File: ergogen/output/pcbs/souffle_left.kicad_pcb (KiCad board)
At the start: 2 copper layers, 135.6 x 116.1 mm, 60 parts

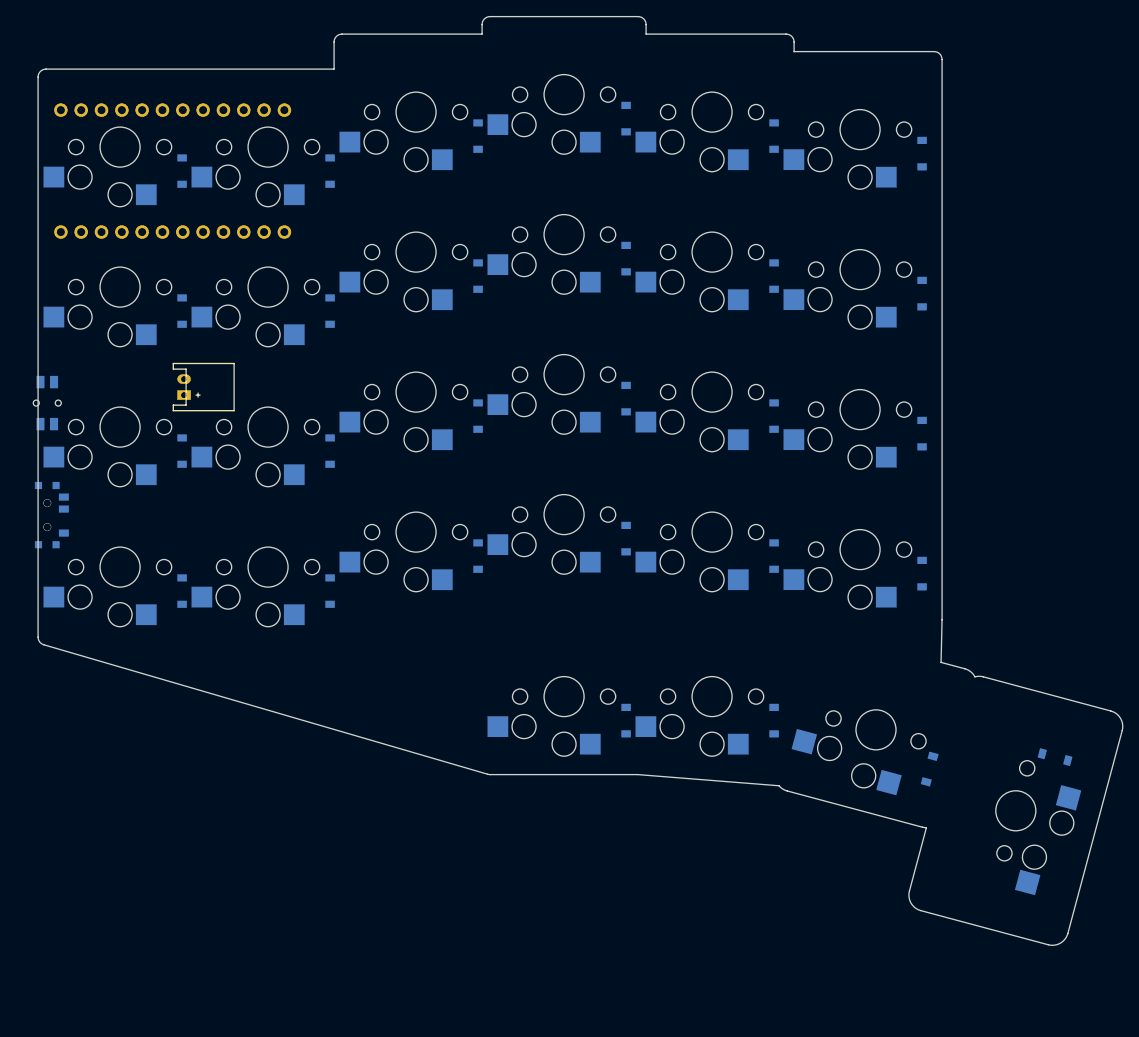
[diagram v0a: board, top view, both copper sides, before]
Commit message: feat: left hand redesign
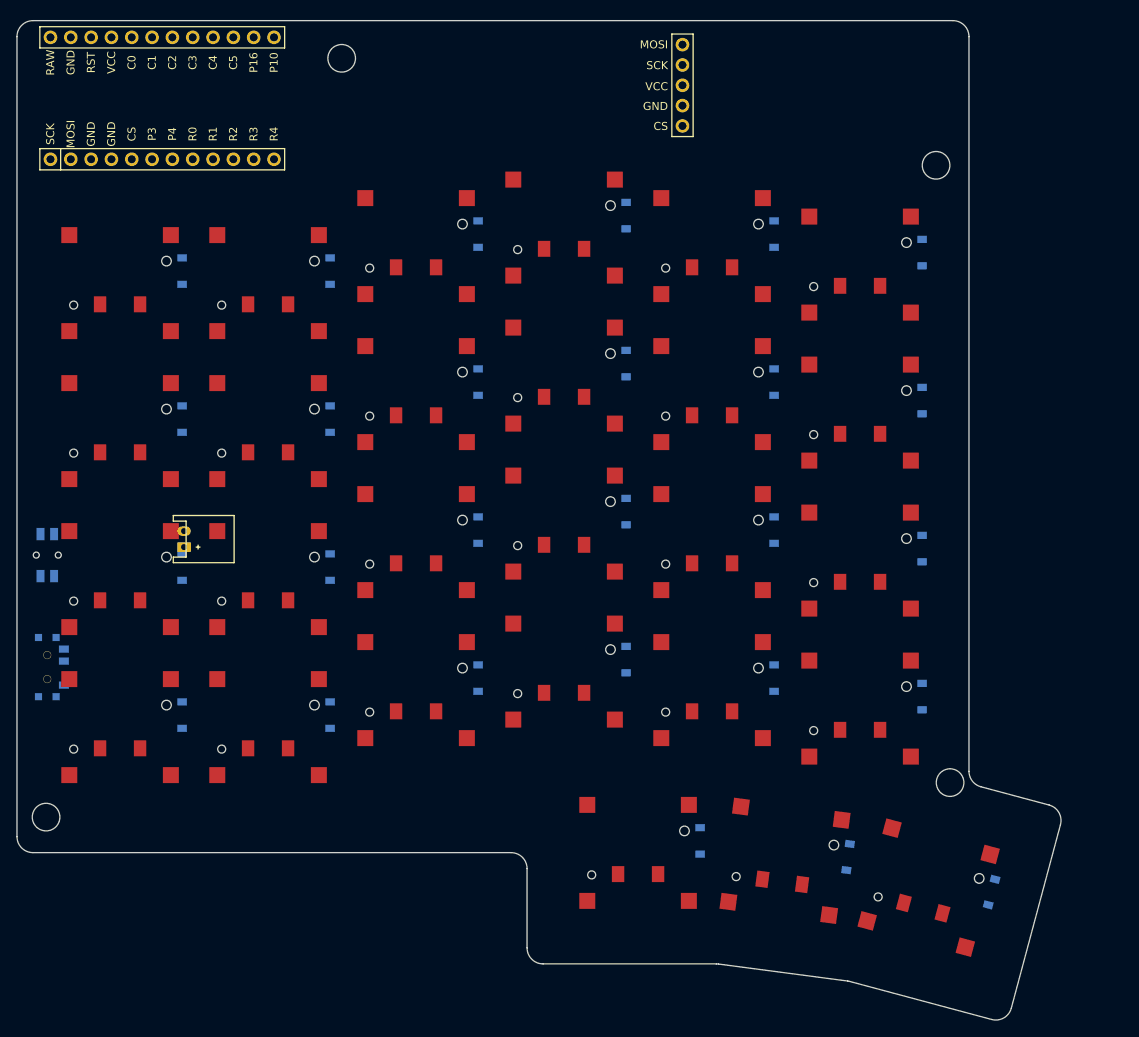
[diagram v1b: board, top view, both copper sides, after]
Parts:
- removed D28: , ceoloide:diode_tht_sod123
- removed S28: , ceoloide:switch_choc_v1_v2
- added DISP1: , ceoloide:display_nice_view, F.Cu at (187.0, 39.8)
- added MH1: , ceoloide:mounting_hole_npth, F.Cu at (127.7, 36.4)
- added MH2: , ceoloide:mounting_hole_npth, F.Cu at (202.0, 49.8)
- added MH3: , ceoloide:mounting_hole_npth, F.Cu at (90.8, 131.2)
- added MH4: , ceoloide:mounting_hole_npth, F.Cu at (203.8, 126.9)
- MCU1: moved to F.Cu
- S1, S10, S11, S12, S13, S14, S15, S16, S17, S18, S19, S2, S20, S21, S22, S23, S24, S25, S26, S27, S3, S4, S5, S6, S7, S8, S9: footprint ceoloide:switch_choc_v1_v2 -> CPG1316S01D02_mikeholscher; moved to F.Cu
- moved S26 22.5 mm to (183.1, 136.7), turned to -7.5 degrees
- moved S25 21.6 mm to (164.8, 135.7), turned to 0 degrees
- moved S27 20.8 mm to (201.1, 140.1), turned to -15 degrees
- moved S1 20.0 mm to (100.0, 120.0), turned to 0 degrees
- moved S5 20.0 mm to (118.5, 120.0), turned to 0 degrees
- moved S21 19.9 mm to (192.5, 117.7), turned to 0 degrees
- moved S17 19.8 mm to (174.0, 115.4), turned to 0 degrees
- moved S9 19.8 mm to (137.0, 115.4), turned to 0 degrees
- moved S13 19.6 mm to (155.5, 113.1), turned to 0 degrees
- moved D26 19.4 mm to (191.0, 136.2), turned to 82.5 degrees
- moved B1 19.0 mm to (90.9, 98.5)
- moved JST1 19.0 mm to (108.0, 96.5)
- moved S2 19.0 mm to (100.0, 101.5), turned to 0 degrees
- moved S6 19.0 mm to (118.5, 101.5), turned to 0 degrees
- moved T1 19.0 mm to (90.9, 112.5)
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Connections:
- D26 pad 2: outward_home -> middle_home
- D27 pad 2: small_thumbkey_home -> outward_home
- MCU1 pad 1: LED -> RAW
- MCU1 pad 10: R2 -> C5
- MCU1 pad 11: R3 -> P16
- MCU1 pad 12: P9 -> P10
- MCU1 pad 13: P10 -> R4
- MCU1 pad 14: P16 -> R3
- MCU1 pad 15: C5 -> R2
- MCU1 pad 16: C4 -> R1
- MCU1 pad 17: C3 -> R0
- MCU1 pad 18: C2 -> P4
- MCU1 pad 19: C1 -> P3
- MCU1 pad 2: DAT -> GND
- MCU1 pad 20: C0 -> CS
- MCU1 pad 21: VCC -> GND
- MCU1 pad 22: RST -> GND
- MCU1 pad 23: GND -> MOSI
- MCU1 pad 24: RAW -> SCK
- MCU1 pad 3: GND -> RST
- MCU1 pad 4: GND -> VCC
- MCU1 pad 5: SDA -> C0
- MCU1 pad 6: SCL -> C1
- MCU1 pad 7: CS -> C2
- MCU1 pad 8: R0 -> C3
- MCU1 pad 9: R1 -> C4
- S1 pad 1: C0 -> outer_bottom
- S1 pad 2: outer_bottom -> C0
- S10 pad 1: C2 -> ring_home
- S10 pad 2: ring_home -> C2
- S11 pad 1: C2 -> ring_top
- S11 pad 2: ring_top -> C2
- S12 pad 1: C2 -> ring_number
- S12 pad 2: ring_number -> C2
- S13 pad 1: C3 -> middle_bottom
- S13 pad 2: middle_bottom -> C3
- S14 pad 1: C3 -> middle_home
- S14 pad 2: middle_home -> C3
- S15 pad 1: C3 -> middle_top
- S15 pad 2: middle_top -> C3
- S16 pad 1: C3 -> middle_number
- S16 pad 2: middle_number -> C3
- S17 pad 1: C4 -> index_bottom
- S17 pad 2: index_bottom -> C4
- S18 pad 1: C4 -> index_home
- S18 pad 2: index_home -> C4
- S19 pad 1: C4 -> index_top
- S19 pad 2: index_top -> C4
- S2 pad 1: C0 -> outer_home
- S2 pad 2: outer_home -> C0
- S20 pad 1: C4 -> index_number
- S20 pad 2: index_number -> C4
- S21 pad 1: C5 -> inner_bottom
- S21 pad 2: inner_bottom -> C5
- S22 pad 1: C5 -> inner_home
- S22 pad 2: inner_home -> C5
- S23 pad 1: C5 -> inner_top
- S23 pad 2: inner_top -> C5
- S24 pad 1: C5 -> inner_number
- S24 pad 2: inner_number -> C5
- S25 pad 1: C2 -> inward_home
- S25 pad 2: inward_home -> C2
- S26 pad 1: C3 -> middle_home
- S26 pad 2: outward_home -> C4
- S27 pad 1: C4 -> outward_home
- S27 pad 2: small_thumbkey_home -> C5
- S3 pad 1: C0 -> outer_top
- S3 pad 2: outer_top -> C0
- S4 pad 1: C0 -> outer_number
- S4 pad 2: outer_number -> C0
- S5 pad 1: C1 -> pinky_bottom
- S5 pad 2: pinky_bottom -> C1
- S6 pad 1: C1 -> pinky_home
- S6 pad 2: pinky_home -> C1
- S7 pad 1: C1 -> pinky_top
- S7 pad 2: pinky_top -> C1
- S8 pad 1: C1 -> pinky_number
- S8 pad 2: pinky_number -> C1
- S9 pad 1: C2 -> ring_bottom
- S9 pad 2: ring_bottom -> C2
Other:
- board size 135.6 x 116.1 mm -> 130.5 x 124.9 mm

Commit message: feat: attempt to move mcu to bottom
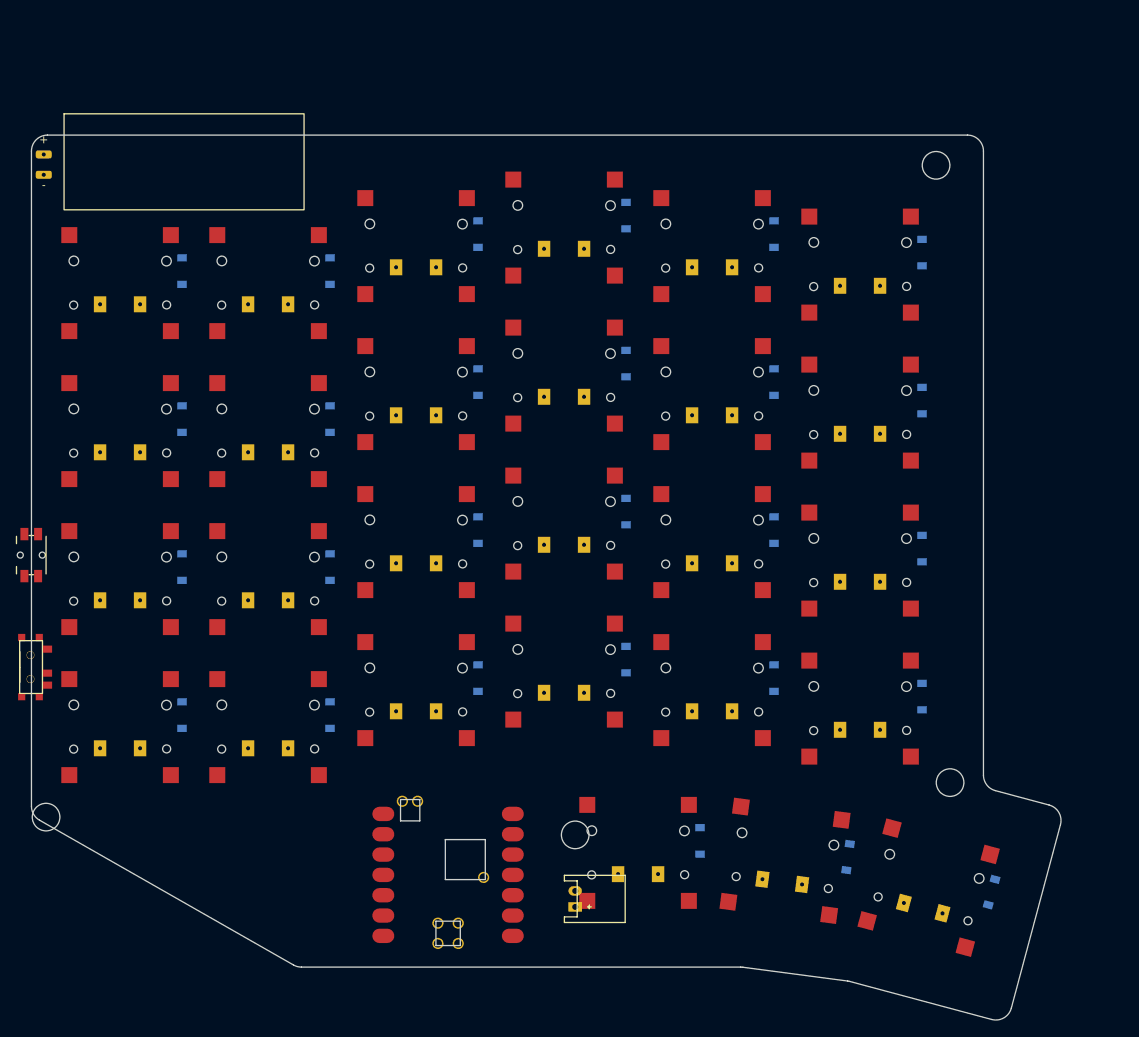
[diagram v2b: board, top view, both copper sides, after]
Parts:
- removed DISP1: , ceoloide:display_nice_view
- added BAT1: , lipo-reversible, F.Cu at (93.0, 53.5)
- MCU1: footprint ceoloide:mcu_nice_nano -> xiao_smd
- S1, S10, S11, S12, S13, S14, S15, S16, S17, S18, S19, S2, S20, S21, S22, S23, S24, S25, S26, S27, S3, S4, S5, S6, S7, S8, S9: footprint CPG1316S01D02_mikeholscher -> CPG1316S01D02
- moved MCU1 103.9 mm to (141.0, 138.5), turned to 180 degrees
- moved MH1 101.4 mm to (156.9, 133.5)
- moved JST1 66.4 mm to (156.9, 141.5)
- moved T1 2.10 mm to (88.8, 112.5)
- moved B1 2.00 mm to (88.9, 98.5)
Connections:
- net P10 renamed RAW3V3
- net P3 renamed BAT
- MCU1 pad 1: RAW -> R0
- MCU1 pad 10: C5 -> C4
- MCU1 pad 11: P16 -> C5
- MCU1 pad 13: R4 -> GND
- MCU1 pad 14: R3 -> RAW5V
- MCU1 pad 15: R2 -> CLK
- MCU1 pad 16: R1 -> DIO
- MCU1 pad 17: R0 -> RST
- MCU1 pad 18: P4 -> GND
- MCU1 pad 2: GND -> R1
- MCU1 pad 20: CS -> NFC1
- MCU1 pad 21: GND -> NFC2
- MCU1 pad 3: RST -> R2
- MCU1 pad 4: VCC -> R3
- MCU1 pad 5: C0 -> R4
- MCU1 pad 6: C1 -> C0
- MCU1 pad 7: C2 -> C1
- MCU1 pad 8: C3 -> C2
- MCU1 pad 9: C4 -> C3
- S1 pad 1: outer_bottom -> C0
- S1 pad 2: C0 -> outer_bottom
- S10 pad 1: ring_home -> C2
- S10 pad 2: C2 -> ring_home
- S11 pad 1: ring_top -> C2
- S11 pad 2: C2 -> ring_top
- S12 pad 1: ring_number -> C2
- S12 pad 2: C2 -> ring_number
- S13 pad 1: middle_bottom -> C3
- S13 pad 2: C3 -> middle_bottom
- S14 pad 1: middle_home -> C3
- S14 pad 2: C3 -> middle_home
- S15 pad 1: middle_top -> C3
- S15 pad 2: C3 -> middle_top
- S16 pad 1: middle_number -> C3
- S16 pad 2: C3 -> middle_number
- S17 pad 1: index_bottom -> C4
- S17 pad 2: C4 -> index_bottom
- S18 pad 1: index_home -> C4
- S18 pad 2: C4 -> index_home
- S19 pad 1: index_top -> C4
- S19 pad 2: C4 -> index_top
- S2 pad 1: outer_home -> C0
- S2 pad 2: C0 -> outer_home
- S20 pad 1: index_number -> C4
- S20 pad 2: C4 -> index_number
- S21 pad 1: inner_bottom -> C5
- S21 pad 2: C5 -> inner_bottom
- S22 pad 1: inner_home -> C5
- S22 pad 2: C5 -> inner_home
- S23 pad 1: inner_top -> C5
- S23 pad 2: C5 -> inner_top
- S24 pad 1: inner_number -> C5
- S24 pad 2: C5 -> inner_number
- S25 pad 1: inward_home -> C3
- S25 pad 2: C2 -> inward_home
- S26 pad 1: middle_home -> C4
- S26 pad 2: C4 -> middle_home
- S27 pad 1: outward_home -> C5
- S27 pad 2: C5 -> outward_home
- S3 pad 1: outer_top -> C0
- S3 pad 2: C0 -> outer_top
- S4 pad 1: outer_number -> C0
- S4 pad 2: C0 -> outer_number
- S5 pad 1: pinky_bottom -> C1
- S5 pad 2: C1 -> pinky_bottom
- S6 pad 1: pinky_home -> C1
- S6 pad 2: C1 -> pinky_home
- S7 pad 1: pinky_top -> C1
- S7 pad 2: C1 -> pinky_top
- S8 pad 1: pinky_number -> C1
- S8 pad 2: C1 -> pinky_number
- S9 pad 1: ring_bottom -> C2
- S9 pad 2: C2 -> ring_bottom
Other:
- board size 130.5 x 124.9 mm -> 128.7 x 110.6 mm
